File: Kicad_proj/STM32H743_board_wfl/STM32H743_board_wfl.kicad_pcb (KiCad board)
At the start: 4 copper layers, 38.5 x 38.5 mm, 64 parts, among them J1 GPS, J2 ESC, J3 UART, J4 Tag_Connect_6pin, U1 LT8609SEV#PBF, U2 AP7361C-33E, U3 STM32H743VITx, U4 W25Q512JVEIQ, U5 BMI088, Y1 TSX-3225_16.0000MF18X-AC0

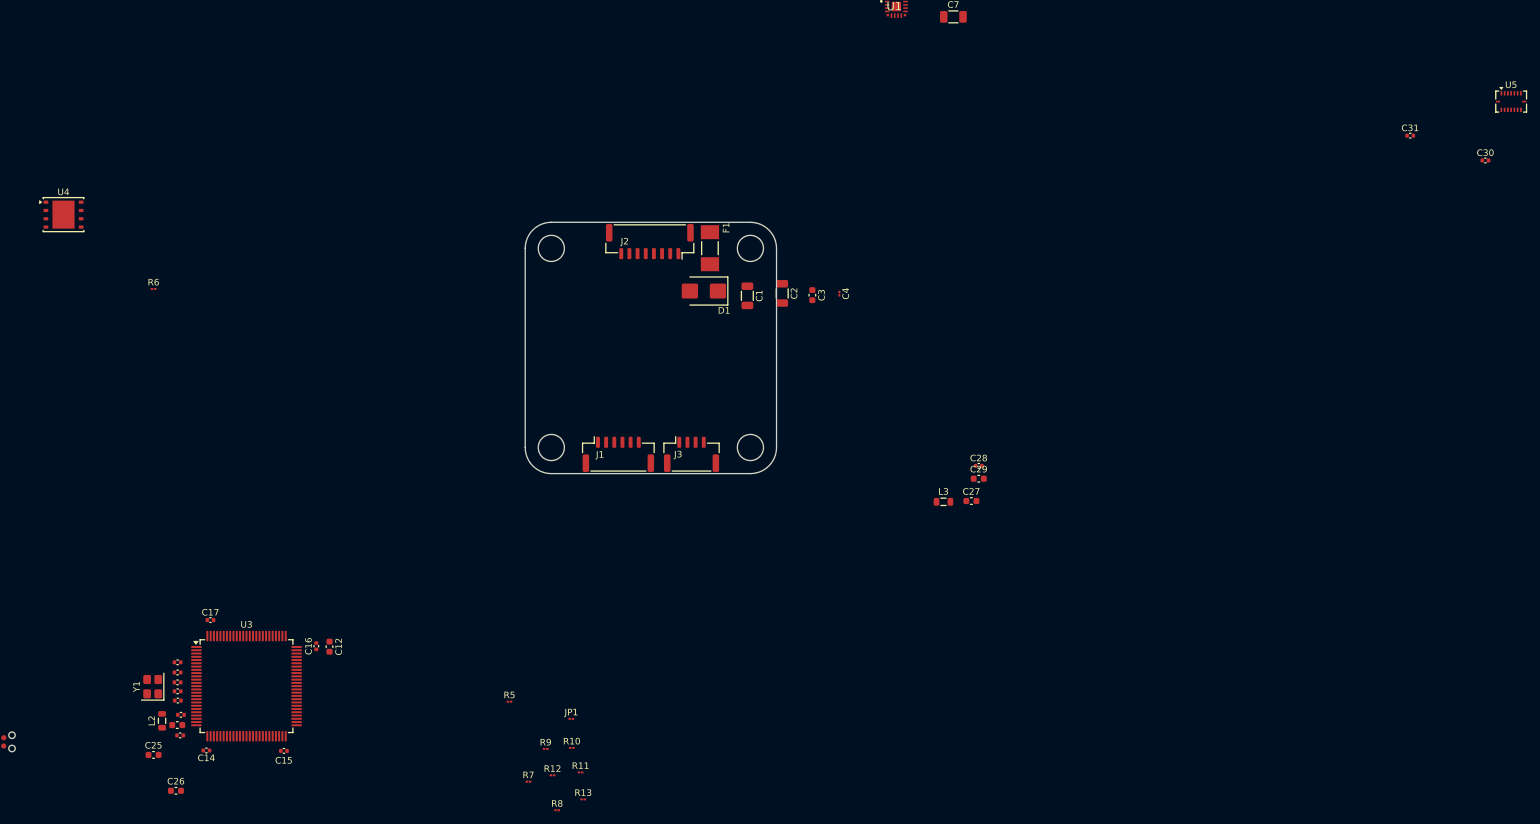
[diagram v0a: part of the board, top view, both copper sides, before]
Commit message: PCB v0.2 STM32 components preplaced
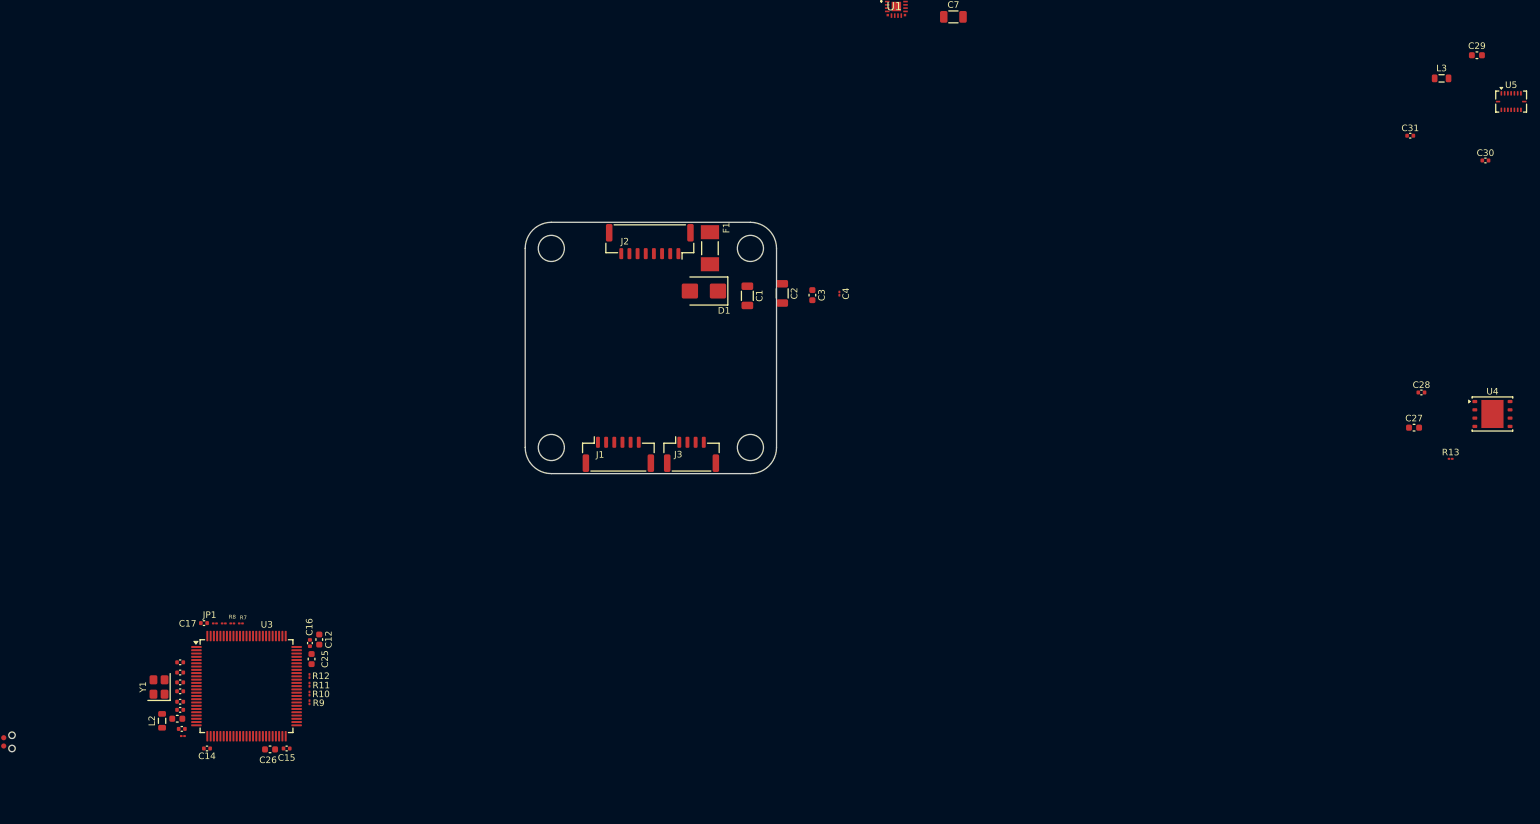
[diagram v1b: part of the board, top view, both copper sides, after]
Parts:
- moved U4 221.0 mm to (248.2, 129.4)
- moved R13 142.8 mm to (241.8, 136.2)
- moved C29 100.2 mm to (245.8, 74.4)
- moved L3 100.2 mm to (240.4, 78.0)
- moved C27 68.7 mm to (236.2, 131.5)
- moved C28 68.7 mm to (237.3, 126.1)
- moved R8 57.4 mm to (55.1, 161.4)
- moved JP1 56.5 mm to (52.5, 161.4), turned to 180 degrees
- moved R6 52.4 mm to (53.8, 161.4)
- moved R5 50.3 mm to (47.6, 178.7)
- moved R7 50.3 mm to (56.4, 161.4), turned to 180 degrees
- moved R11 43.7 mm to (67.0, 170.8), turned to -90 degrees
- moved R10 41.0 mm to (67.0, 172.2), turned to -90 degrees
- moved R12 40.2 mm to (67.0, 169.5), turned to -90 degrees
- moved R9 36.9 mm to (67.0, 173.5), turned to -90 degrees
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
